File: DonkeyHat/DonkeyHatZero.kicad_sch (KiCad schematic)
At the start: 17 parts, among them J1 GPIO, J2 Encoder 2, J3 Encoder 1, J4 I2C, J5 Battery +, J6 Battery -, J7 +5v, J8 GND, U2 rp2040-zero

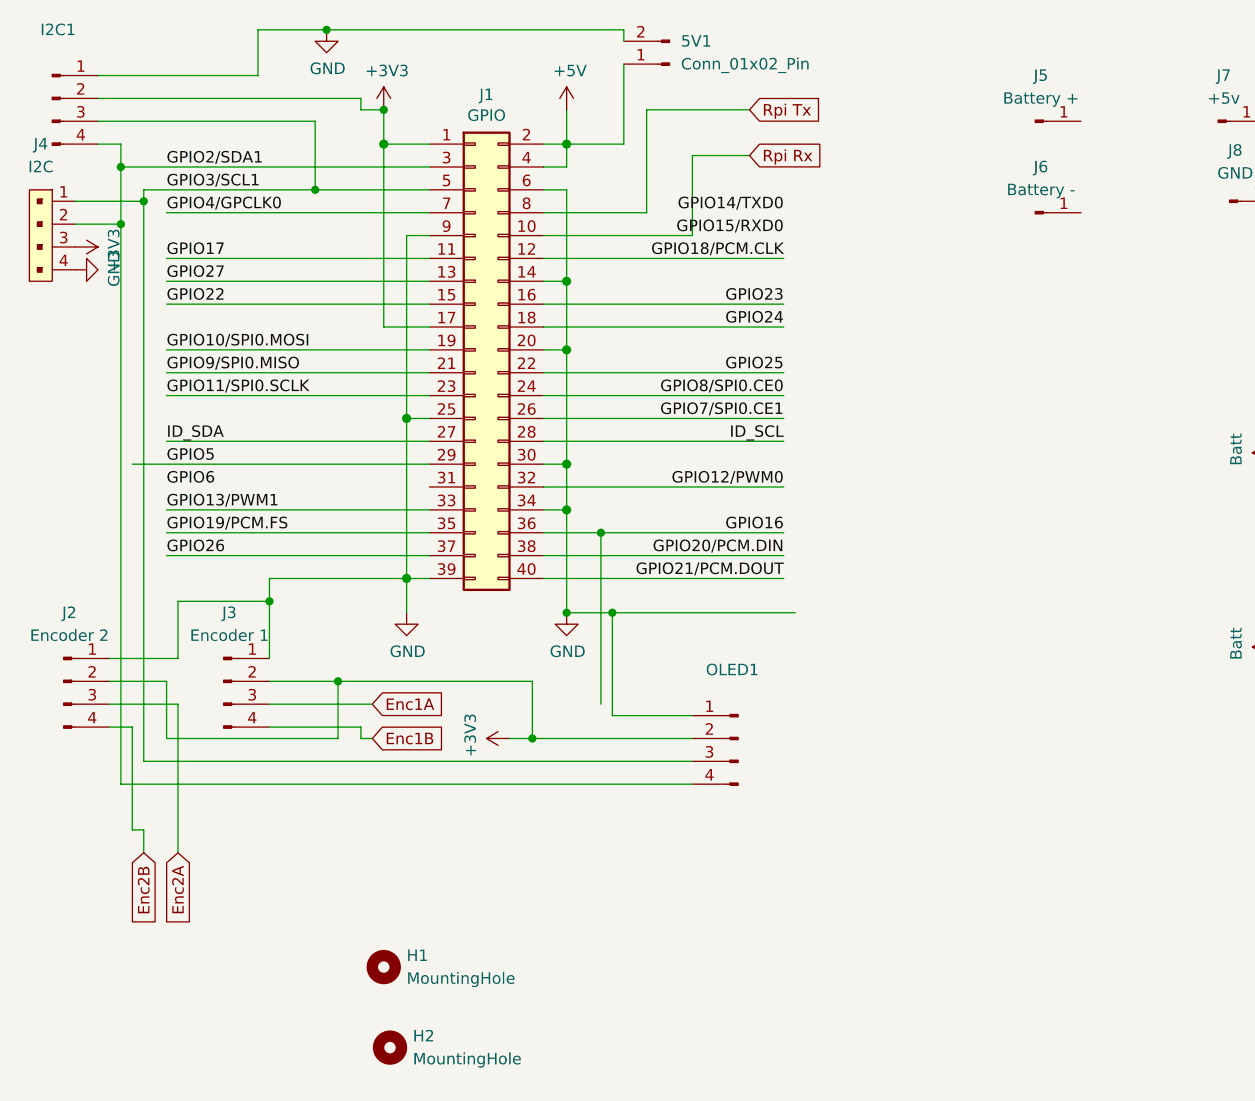
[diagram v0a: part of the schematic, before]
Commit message: Zero WIP
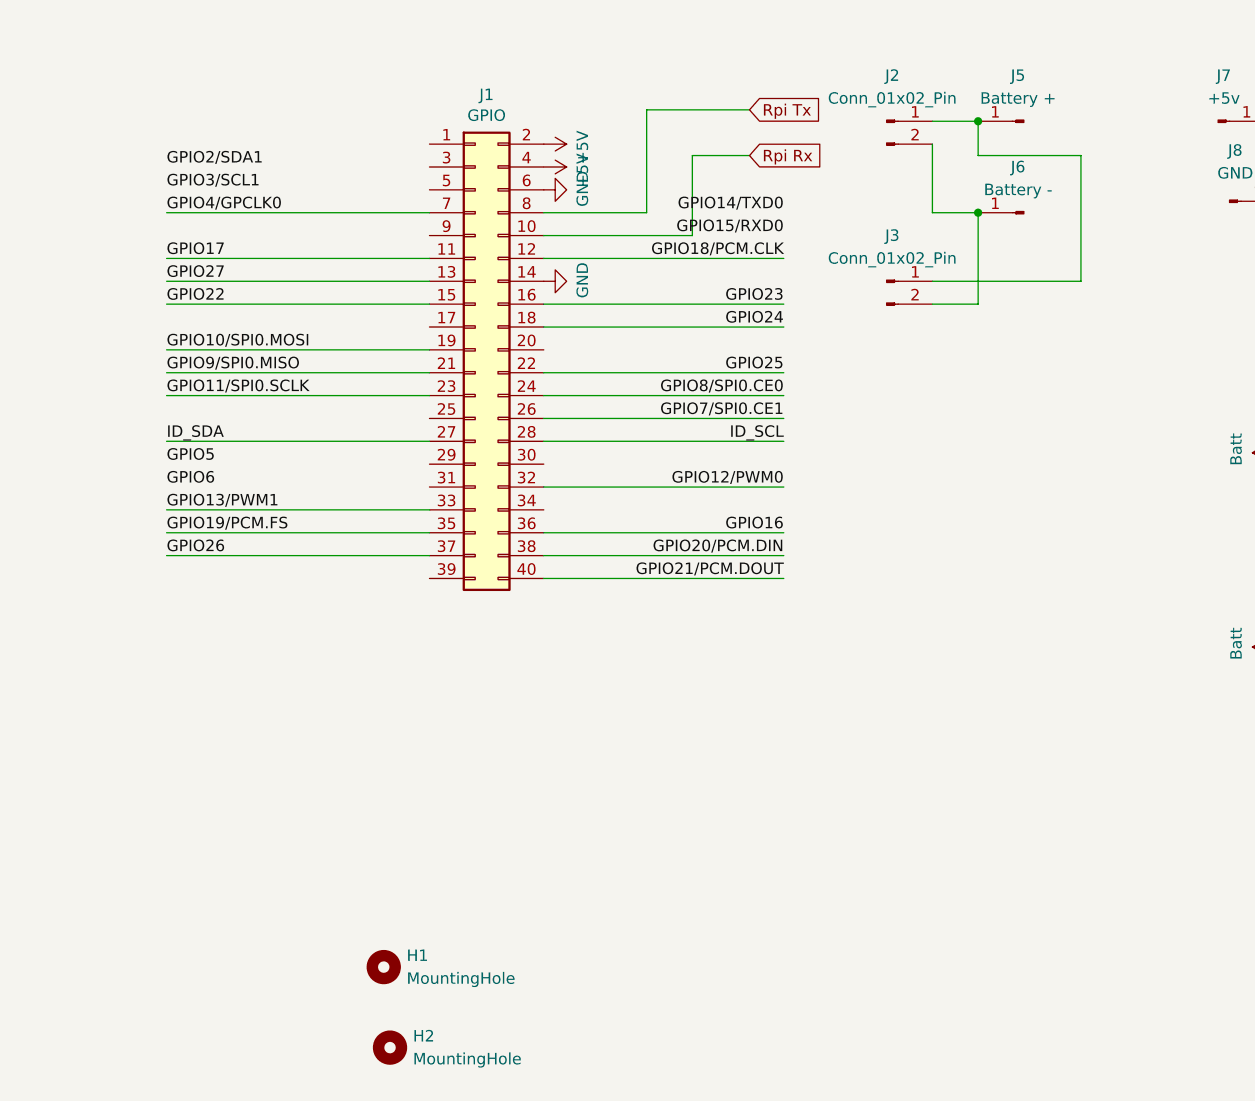
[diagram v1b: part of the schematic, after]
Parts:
- removed 5V1: Conn_01x02_Pin, Connector_PinHeader_2.54mm:PinHeader_1x02_P2.54mm_Vertical, symbol Connector:Conn_01x02_Pin
- removed I2C1, OLED1: Conn_01x04_Pin, Connector_PinHeader_2.54mm:PinHeader_1x04_P2.54mm_Vertical, symbol Connector:Conn_01x04_Pin
- removed J2: Encoder 2, Connector_PinHeader_2.54mm:PinHeader_1x04_P2.54mm_Vertical, symbol Connector:Conn_01x04_Pin
- removed J3: Encoder 1, Connector_PinHeader_2.54mm:PinHeader_1x04_P2.54mm_Vertical, symbol Connector:Conn_01x04_Pin
- removed J4: I2C, Connector_JST:JST_SH_BM04B-SRSS-TB_1x04-1MP_P1.00mm_Vertical, symbol dk_Rectangular-Connectors-Headers-Male-Pins:B4B-PH-K-S_LF__SN_
- added J2, J3: Conn_01x02_Pin, Connector_PinHeader_2.54mm:PinHeader_1x02_P2.54mm_Vertical, symbol Connector:Conn_01x02_Pin
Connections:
- net GND: no longer J1.20 (Pin_20), J1.25 (Pin_25), J1.30 (Pin_30), J1.34 (Pin_34), J1.39 (Pin_39), J1.9 (Pin_9)
- net GPIO2/SDA1: no longer J1.3 (Pin_3)
- net GPIO3/SCL1: no longer J1.5 (Pin_5)
- net GPIO5: no longer J1.29 (Pin_29)
- net at J6.1 (Pin_1): now also J2.2 (Pin_2), J3.2 (Pin_2)
- net at J5.1 (Pin_1): now also J2.1 (Pin_1), J3.1 (Pin_1)
- net +3V3: no longer names the net of J1.1 (Pin_1)
- net +3V3: no longer J1.17 (Pin_17)
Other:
- moved on the sheet: J5, J6
